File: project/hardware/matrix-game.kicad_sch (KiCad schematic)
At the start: 31 parts, among them SW1 button_center, SW2 button_left, SW3 button_down, SW4 button_right, SW5 button_up, U1 NUCLEO-F042K6, U2 MAX7219, U3 SSD1306

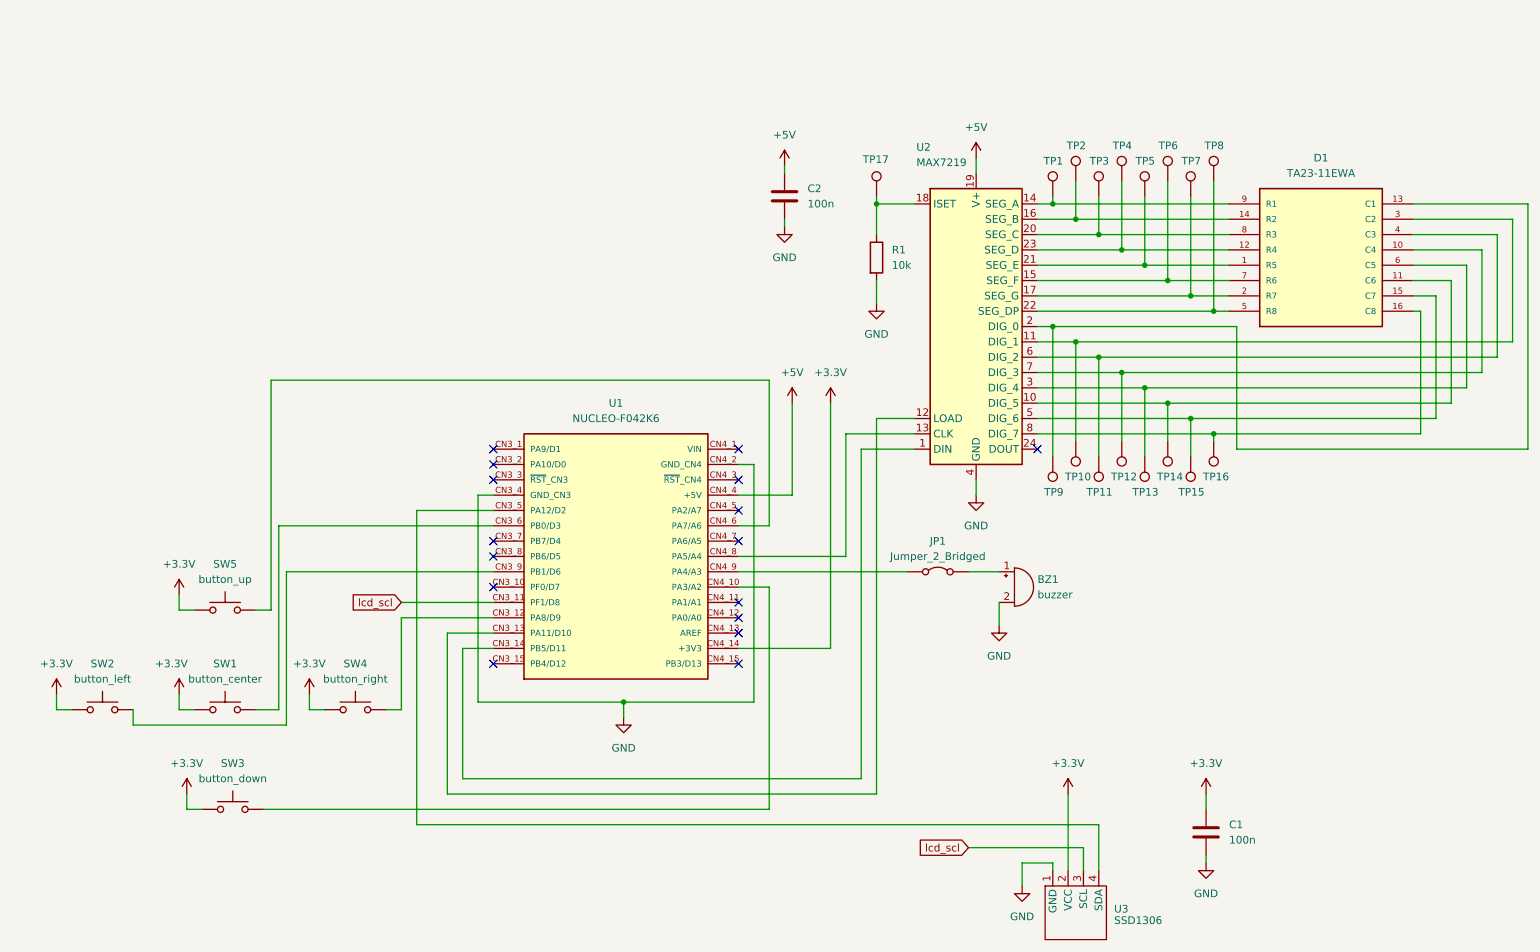
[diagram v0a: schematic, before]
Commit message: [project/hardware/schematic] added labels
Signed-off-by: Timon Burkard <timon.burkard@gwf.ch>
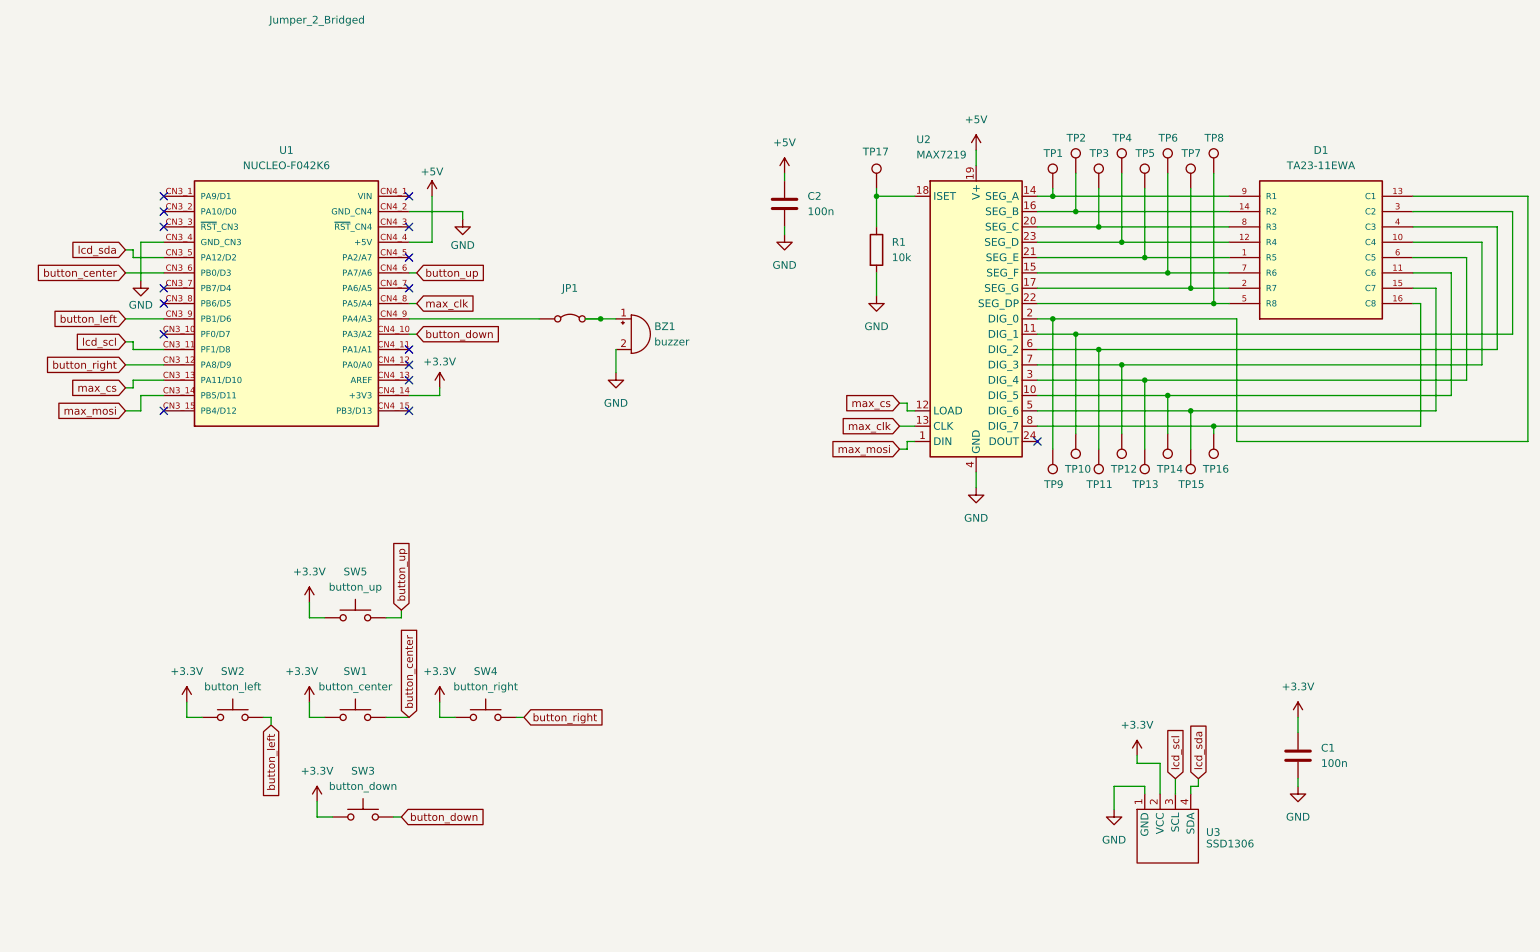
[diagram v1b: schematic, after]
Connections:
- net lcd_sda: now reaches U1.CN3_5 (PA12/D2), U3.4 (SDA)
- net max_mosi: now reaches U1.CN3_14 (PB5/D11), U2.1 (DIN)
- net max_cs: now reaches U1.CN3_13 (PA11/D10), U2.12 (LOAD)
- net max_clk: now reaches U1.CN4_8 (PA5/A4), U2.13 (CLK)
- net button_left: now reaches SW2.2, U1.CN3_9 (PB1/D6)
- net button_right: now reaches SW4.2, U1.CN3_12 (PA8/D9)
- net button_center: now reaches SW1.2, U1.CN3_6 (PB0/D3)
- net button_down: now reaches SW3.2, U1.CN4_10 (PA3/A2)
- net button_up: now reaches SW5.2, U1.CN4_6 (PA7/A6)
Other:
- moved on the sheet: BZ1, C1, C2, D1, JP1, R1, SW1, SW2, SW3, SW4, SW5, TP1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
